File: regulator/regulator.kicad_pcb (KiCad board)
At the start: 2 copper layers, 43 x 10 mm, 10 parts, among them J1 Conn_01x02, J2 Conn_01x02, U1 TPS79333-EP

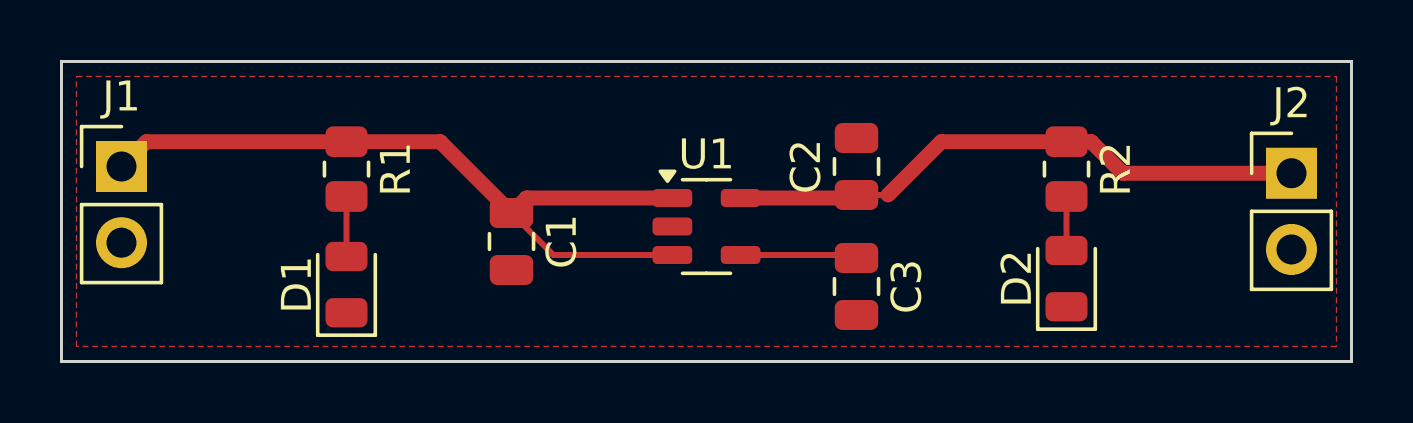
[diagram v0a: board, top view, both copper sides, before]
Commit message: one error
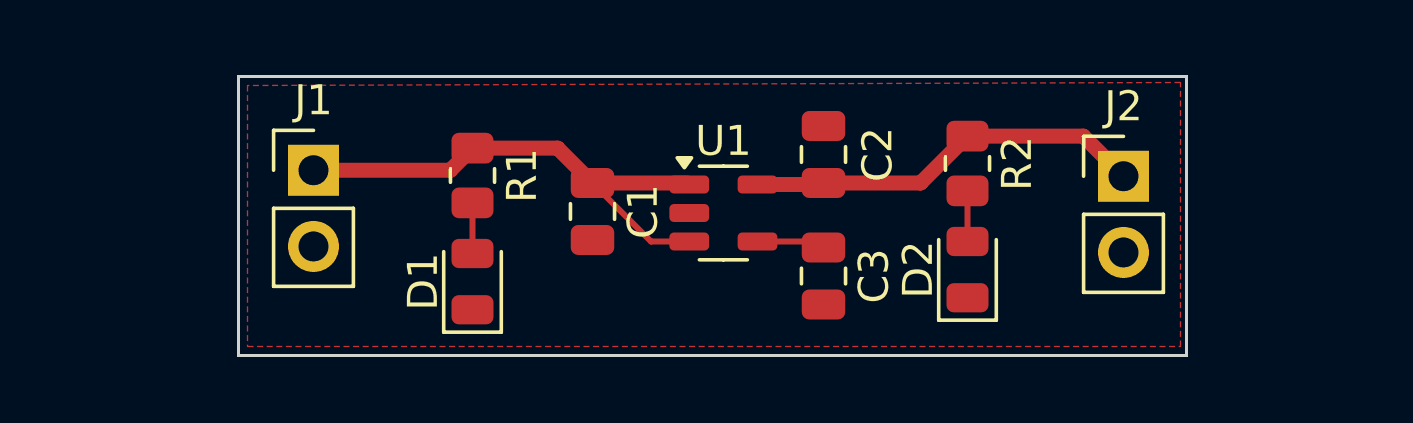
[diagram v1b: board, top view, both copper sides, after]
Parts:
- moved J1 6.40 mm to (131.4, 93.1)
- moved J2 5.60 mm to (158.4, 93.3)
- moved R1 4.21 mm to (136.7, 93.3)
- moved D1 4.20 mm to (136.7, 96.8)
- moved D2 3.31 mm to (153.2, 96.4)
- moved R2 3.31 mm to (153.2, 92.9)
- moved C1 2.88 mm to (140.7, 94.5)
- moved C2 1.17 mm to (148.4, 92.6)
- moved C3 1.15 mm to (148.4, 96.7)
- moved U1 0.72 mm to (145.1, 94.5)
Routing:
- net Net-(J1-Pin_1): track 25.8 -> 17.4 mm
- net Net-(J2-Pin_1): track 19.6 -> 13.4 mm
- net Net-(U1-BP): track 3.90 -> 2.28 mm
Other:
- board size 43 x 10 mm -> 31.6 x 9.3 mm
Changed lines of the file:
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@@
 	(footprint "Connector_PinHeader_2.54mm:PinHeader_1x02_P2.54mm_Vertical"
 		(layer "F.Cu")
-		(at 164 93.225)
+		(at 158.4 93.325)
 		(descr "Through hole straight pin header, 1x02, 2.54mm pitch, single row")
 		(tags "Through hole pin header THT 1x02 2.54mm single row")
@@
 	(footprint "Resistor_SMD:R_0805_2012Metric"
 		(layer "F.Cu")
-		(at 156.5 93.0875 -90)
+		(at 153.2 92.9 -90)
 		(descr "Resistor SMD 0805 (2012 Metric), square (rectangular) end terminal, IPC_7351 nominal, (Body size source: IPC-SM-782 page 72, https://www.pcb-3d.com/wordpress/wp-content/uploads/ipc-sm-782a_amendment_1_and_2.pdf), generated with kicad-footprint-generator")
 		(tags "resistor")
@@
 	(footprint "Connector_PinHeader_2.54mm:PinHeader_1x02_P2.54mm_Vertical"
 		(layer "F.Cu")
-		(at 125 93)
+		(at 131.4 93.125)
 		(descr "Through hole straight pin header, 1x02, 2.54mm pitch, single row")
 		(tags "Through hole pin header THT 1x02 2.54mm single row")
@@
 			(pinfunction "Pin_2")
 			(pintype "passive")
+			(zone_connect 2)
 		)
 		(model "${KICAD8_3DMODEL_DIR}/Connector_PinHeader_2.54mm.3dshapes/PinHeader_1x02_P2.54mm_Vertical.wrl"
@@
 	(footprint "Capacitor_SMD:C_0805_2012Metric"
 		(layer "F.Cu")
-		(at 149.5 93 90)
+		(at 148.4 92.6 90)
 		(descr "Capacitor SMD 0805 (2012 Metric), square (rectangular) end terminal, IPC_7351 nominal, (Body size source: IPC-SM-782 page 76, https://www.pcb-3d.com/wordpress/wp-content/uploads/ipc-sm-782a_amendment_1_and_2.pdf, https://docs.google.com/spreadsheets/d/1BsfQQcO9C6DZCsRaXUlFlo91Tg2WpOkGARC1WS5S8t0/edit?usp=sharing), generated with kicad-footprint-generator")
 		(tags "capacitor")
 		(property "Reference" "C2"
-			(at 0 -1.68 90)
+			(at 0 1.8 90)
 			(layer "F.SilkS")
 			(effects
@@
 	(footprint "Resistor_SMD:R_0805_2012Metric"
 		(layer "F.Cu")
-		(at 132.5 93.0875 -90)
+		(at 136.7 93.3 -90)
 		(descr "Resistor SMD 0805 (2012 Metric), square (rectangular) end terminal, IPC_7351 nominal, (Body size source: IPC-SM-782 page 72, https://www.pcb-3d.com/wordpress/wp-content/uploads/ipc-sm-782a_amendment_1_and_2.pdf), generated with kicad-footprint-generator")
 		(tags "resistor")
@@
 	(footprint "LED_SMD:LED_0805_2012Metric"
 		(layer "F.Cu")
-		(at 132.5 96.9375 90)
+		(at 136.7 96.8375 90)
 		(descr "LED SMD 0805 (2012 Metric), square (rectangular) end terminal, IPC_7351 nominal, (Body size source: https://docs.google.com/spreadsheets/d/1BsfQQcO9C6DZCsRaXUlFlo91Tg2WpOkGARC1WS5S8t0/edit?usp=sharing), generated with kicad-footprint-generator")
 		(tags "LED")
@@
 			(pinfunction "K")
 			(pintype "passive")
+			(zone_connect 2)
 		)
 		(pad "2" smd roundrect
@@
 	(footprint "LED_SMD:LED_0805_2012Metric"
 		(layer "F.Cu")
-		(at 156.5 96.7375 90)
+		(at 153.2 96.4375 90)
 		(descr "LED SMD 0805 (2012 Metric), square (rectangular) end terminal, IPC_7351 nominal, (Body size source: https://docs.google.com/spreadsheets/d/1BsfQQcO9C6DZCsRaXUlFlo91Tg2WpOkGARC1WS5S8t0/edit?usp=sharing), generated with kicad-footprint-generator")
 		(tags "LED")
@@
 	(footprint "Capacitor_SMD:C_0805_2012Metric"
 		(layer "F.Cu")
-		(at 149.5 97 -90)
+		(at 148.4 96.65 -90)
 		(descr "Capacitor SMD 0805 (2012 Metric), square (rectangular) end terminal, IPC_7351 nominal, (Body size source: IPC-SM-782 page 76, https://www.pcb-3d.com/wordpress/wp-content/uploads/ipc-sm-782a_amendment_1_and_2.pdf, https://docs.google.com/spreadsheets/d/1BsfQQcO9C6DZCsRaXUlFlo91Tg2WpOkGARC1WS5S8t0/edit?usp=sharing), generated with kicad-footprint-generator")
 		(tags "capacitor")
@@
 	(footprint "Capacitor_SMD:C_0805_2012Metric"
 		(layer "F.Cu")
-		(at 138 95.5 -90)
+		(at 140.7 94.5 -90)
 		(descr "Capacitor SMD 0805 (2012 Metric), square (rectangular) end terminal, IPC_7351 nominal, (Body size source: IPC-SM-782 page 76, https://www.pcb-3d.com/wordpress/wp-content/uploads/ipc-sm-782a_amendment_1_and_2.pdf, https://docs.google.com/spreadsheets/d/1BsfQQcO9C6DZCsRaXUlFlo91Tg2WpOkGARC1WS5S8t0/edit?usp=sharing), generated with kicad-footprint-generator")
 		(tags "capacitor")
@@
 	(footprint "Package_TO_SOT_SMD:SOT-23-5"
 		(layer "F.Cu")
-		(at 144.5 95)
+		(at 145.0625 94.55)
 		(descr "SOT, 5 Pin (JEDEC MO-178 Var AA https://www.jedec.org/document_search?search_api_views_fulltext=MO-178), generated with kicad-footprint-generator ipc_gullwing_generator.py")
 		(tags "SOT TO_SOT_SMD")
@@
 	)
 	(gr_rect
-		(start 123 89.5)
-		(end 166 99.5)
+		(start 128.9 90)
+		(end 160.5 99.3)
 		(stroke
 			(width 0.1)
@@
 	)
 	(segment
-		(start 138.5 94.05)
-		(end 143.3625 94.05)
+		(start 142.65 95.5)
+		(end 140.7 93.55)
+		(width 0.2)
+		(layer "F.Cu")
+		(net 2)
+	)
+	(segment
+		(start 131.4 93.125)
+		(end 135.9625 93.125)
 		(width 0.5)
 		(layer "F.Cu")
@@
 	)
 	(segment
-		(start 125 93)
-		(end 125.825 92.175)
+		(start 143.875 93.55)
+		(end 143.925 93.6)
+		(width 0.2)
+		(layer "F.Cu")
+		(net 2)
+	)
+	(segment
+		(start 135.9625 93.125)
+		(end 136.7 92.3875)
 		(width 0.5)
 		(layer "F.Cu")
@@
 	)
 	(segment
-		(start 125.825 92.175)
-		(end 132.5 92.175)
+		(start 143.925 95.5)
+		(end 142.65 95.5)
+		(width 0.2)
+		(layer "F.Cu")
+		(net 2)
+	)
+	(segment
+		(start 139.5375 92.3875)
+		(end 140.7 93.55)
 		(width 0.5)
 		(layer "F.Cu")
@@
 	)
 	(segment
-		(start 143.3625 95.95)
-		(end 139.4 95.95)
+		(start 136.7 92.3875)
+		(end 139.5375 92.3875)
+		(width 0.5)
+		(layer "F.Cu")
+		(net 2)
+	)
+	(segment
+		(start 140.7 93.55)
+		(end 143.875 93.55)
+		(width 0.5)
+		(layer "F.Cu")
+		(net 2)
+	)
+	(segment
+		(start 146.2 93.6)
+		(end 148.35 93.6)
+		(width 0.5)
+		(layer "F.Cu")
+		(net 3)
+	)
+	(segment
+		(start 148.35 93.6)
+		(end 148.4 93.55)
 		(width 0.2)
 		(layer "F.Cu")
-		(net 2)
+		(net 3)
 	)
 	(segment
-		(start 138 94.55)
-		(end 138.5 94.05)
+		(start 151.6375 93.55)
+		(end 153.2 91.9875)
 		(width 0.5)
 		(layer "F.Cu")
-		(net 2)
+		(net 3)
 	)
 	(segment
-		(start 135.625 92.175)
-		(end 138 94.55)
+		(start 157.0625 91.9875)
+		(end 158.4 93.325)
 		(width 0.5)
 		(layer "F.Cu")
-		(net 2)
+		(net 3)
 	)
 	(segment
-		(start 132.5 92.175)
-		(end 135.625 92.175)
+		(start 148.4 93.55)
+		(end 151.6375 93.55)
 		(width 0.5)
 		(layer "F.Cu")
-		(net 2)
+		(net 3)
 	)
 	(segment
-		(start 139.4 95.95)
-		(end 138 94.55)
+		(start 153.2 91.9875)
+		(end 157.0625 91.9875)
+		(width 0.5)
+		(layer "F.Cu")
+		(net 3)
+	)
+	(segment
+		(start 148.2 95.5)
+		(end 148.4 95.7)
 		(width 0.2)
 		(layer "F.Cu")
-		(net 2)
+		(net 4)
 	)
 	(segment
-		(start 145.6375 94.05)
-		(end 149.4 94.05)
-		(width 0.5)
-		(layer "F.Cu")
-		(net 3)
+		(start 146.2 95.5)
+		(end 148.2 95.5)
+		(width 0.2)
+		(layer "F.Cu")
+		(net 4)
 	)
 	(segment
-		(start 149.5 93.95)
-		(end 150.55 93.95)
+		(start 136.5 95.7)
+		(end 136.7 95.9)
 		(width 0.2)
 		(layer "F.Cu")
-		(net 3)
+		(net 5)
 	)
 	(segment
-		(start 149.4 94.05)
-		(end 149.5 93.95)
+		(start 136.7 94.2125)
+		(end 136.7 95.9)
 		(width 0.2)
 		(layer "F.Cu")
-		(net 3)
+		(net 5)
 	)
 	(segment
-		(start 152.325 92.175)
-		(end 156.5 92.175)
-		(width 0.5)
-		(layer "F.Cu")
-		(net 3)
-	)
-	(segment
-		(start 150.55 93.95)
-		(end 152.325 92.175)
-		(width 0.5)
-		(layer "F.Cu")
-		(net 3)
-	)
-	(segment
-		(start 156.5 92.175)
-		(end 157.325 92.175)
-		(width 0.5)
-		(layer "F.Cu")
-		(net 3)
-	)
-	(segment
-		(start 157.325 92.175)
-		(end 158.375 93.225)
-		(width 0.5)
-		(layer "F.Cu")
-		(net 3)
-	)
-	(segment
-		(start 158.375 93.225)
-		(end 164 93.225)
-		(width 0.5)
-		(layer "F.Cu")
-		(net 3)
-	)
-	(segment
-		(start 145.6375 95.95)
-		(end 149.4 95.95)
-		(width 0.2)
-		(layer "F.Cu")
-		(net 4)
-	)
-	(segment
-		(start 149.4 95.95)
-		(end 149.5 96.05)
-		(width 0.2)
-		(layer "F.Cu")
-		(net 4)
-	)
-	(segment
-		(start 132.5 94)
-		(end 132.5 96)
-		(width 0.2)
-		(layer "F.Cu")
-		(net 5)
-	)
-	(segment
-		(start 156.5 94)
-		(end 156.5 95.8)
+		(start 153.2 93.8125)
+		(end 153.2 95.5)
 		(width 0.2)
 		(layer "F.Cu")
@@
 		(net_name "GND")
 		(layer "F.Cu")
+		(name "GND")
 		(hatch edge 0.5)
 		(connect_pads yes
@@
 		(polygon
 			(pts
-				(xy 123.5 90) (xy 165.5 90) (xy 165.5 99) (xy 123.5 99)
-			)
-		)
+				(xy 129.2 90.3) (xy 129.2 99) (xy 160.3 99) (xy 160.3 90.2)
+			)
+		)
